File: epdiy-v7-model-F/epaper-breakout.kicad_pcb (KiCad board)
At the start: 4 copper layers, 100 x 55 mm, 111 parts, among them J2 EXTENSION_HEADER, J3 SM04B-SRSS-TB_LF__SN_, J4 XF2M-3315-1A, J5 CONN_BAT, J6 8BIT_HEADER, J7 ESP_HDR, J8 ED133UT2, J9 USB_C_Receptacle_USB2.0, Q1 AO3401A, U1 MCP1700-3302E_SOT23, U10 RT9080-33GJ5, U11 TP4056, U2 PCA9535PW, U3 TPS651851RSLR, U6 ED078KH6, U8 ESP32-S3-WROOM-1, Y1 RV-3032-C7

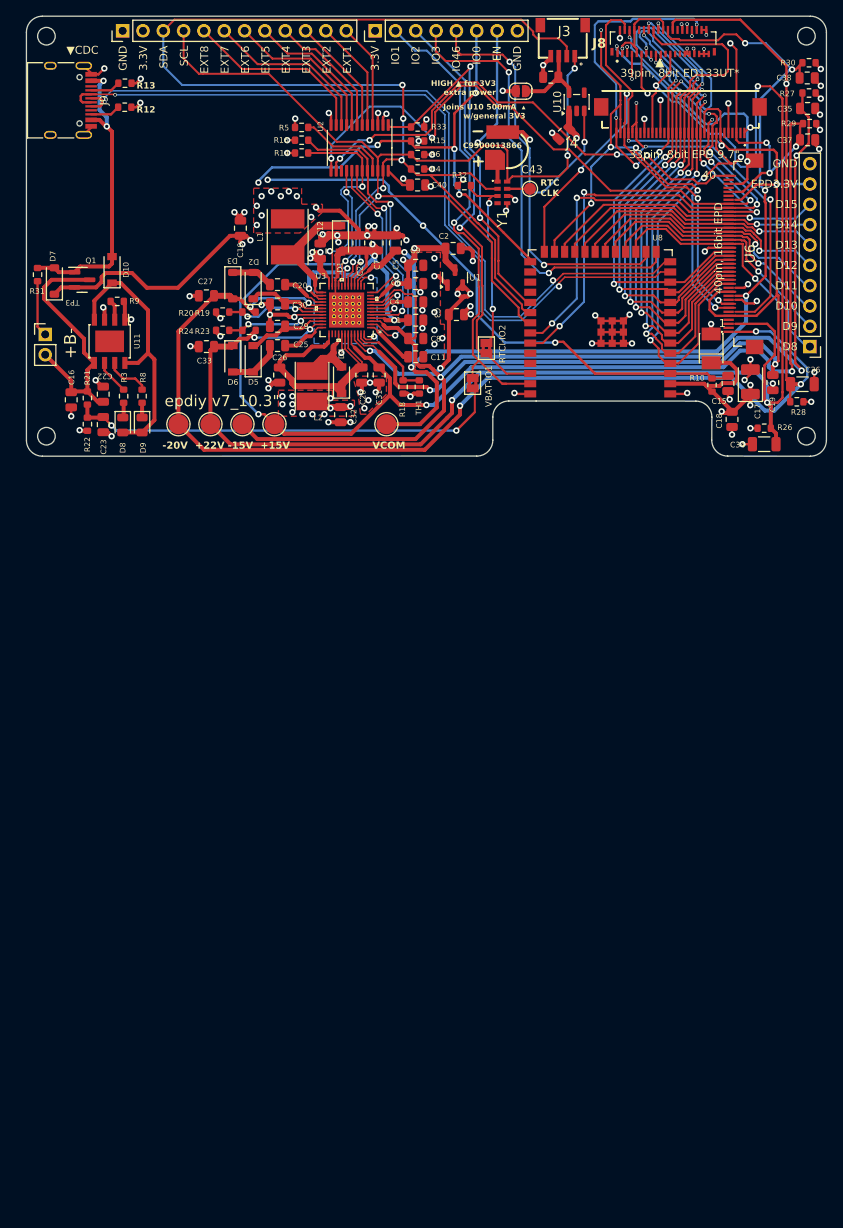
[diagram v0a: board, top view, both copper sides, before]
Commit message: Starting to accomodate stuff over the board
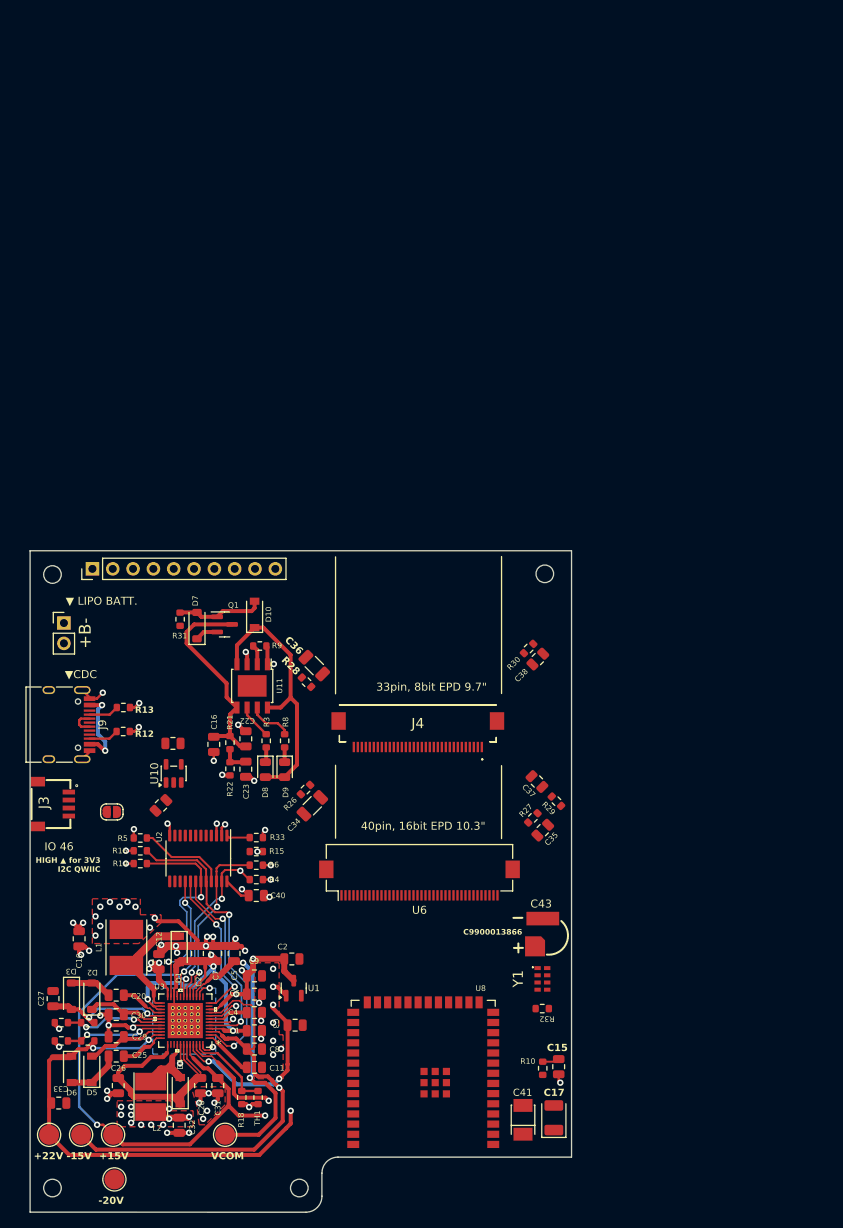
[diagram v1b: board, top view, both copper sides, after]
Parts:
- removed C18: 1uF, Capacitor_SMD:C_0805_2012Metric
- removed C19: 10uF, Capacitor_SMD:C_0805_2012Metric
- removed J2: EXTENSION_HEADER, Connector_PinHeader_2.54mm:PinHeader_1x12_P2.54mm_Vertical
- removed J7: ESP_HDR, Connector_PinHeader_2.54mm:PinHeader_1x08_P2.54mm_Vertical
- removed J8: ED133UT2, epaper-breakout:HRS_FH26W-39S-0.3SHW(60)
- removed JP1: VBAT_GPIO2, Jumper:SolderJumper-2_P1.3mm_Bridged2Bar_Pad1.0x1.5mm
- removed JP2: RTCINT_GPIO2, Jumper:SolderJumper-2_P1.3mm_Bridged2Bar_Pad1.0x1.5mm
- removed TP6: RTC_CLK, TestPoint:TestPoint_Pad_D1.5mm
- U6: footprint footprints:FH1240S05SH55 -> epaper-breakout:Hirose_FH12-40S-0.5SH_mirrored
- moved J3 117.8 mm to (22.5, 115.4), turned to -90 degrees
- moved H3 113.4 mm to (56.0, 166.4)
- moved JP3 103.6 mm to (32.5, 119.4)
- moved R32 103.3 mm to (86.3, 144.0), turned to 0 degrees
- moved C41 99.3 mm to (83.9, 157.9)
- moved Y1 98.4 mm to (86.4, 140.3)
- moved C43 98.4 mm to (85.9, 134.7)
- moved C21 97.9 mm to (38.7, 118.6)
- moved U10 97.9 mm to (40.3, 114.6)
- moved R27 97.0 mm to (85.2, 120.1), turned to 45 degrees
- moved U8 96.4 mm to (71.5, 152.7)
- moved C33 96.3 mm to (25.9, 155.8), turned to 0 degrees
- moved C35 96.1 mm to (86.4, 121.7), turned to 45 degrees
- moved C39 95.7 mm to (40.2, 110.8), turned to 180 degrees
- moved C17 95.2 mm to (87.8, 157.6)
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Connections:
- U2 pad 10: /EXT7 -> unconnected-(U2-IO0_6-Pad10)
- U2 pad 11: /EXT8 -> unconnected-(U2-IO0_7-Pad11)
- U2 pad 4: /EXT1 -> unconnected-(U2-IO0_0-Pad4)
- U2 pad 5: /EXT2 -> unconnected-(U2-IO0_1-Pad5)
- U2 pad 6: /EXT3 -> unconnected-(U2-IO0_2-Pad6)
- U2 pad 7: /EXT4 -> unconnected-(U2-IO0_3-Pad7)
- U2 pad 8: /EXT5 -> unconnected-(U2-IO0_4-Pad8)
- U2 pad 9: /EXT6 -> unconnected-(U2-IO0_5-Pad9)
- U8 pad 10: /D5 -> /D10
- U8 pad 11: /D6 -> /D9
- U8 pad 12: /D7 -> /D8
- U8 pad 17: /D8 -> /D7
- U8 pad 18: /D9 -> /D6
- U8 pad 19: /D10 -> /D5
- U8 pad 20: /D11 -> /D4
- U8 pad 21: /D12 -> /D3
- U8 pad 22: /D13 -> /D2
- U8 pad 23: /D14 -> /D1
- U8 pad 24: /D15 -> /D0
- U8 pad 25: /CKV -> /LEH
- U8 pad 26: /EP_STV -> /XSTL
- U8 pad 31: /~{GPIO_INTR} -> /GPIO_38
- U8 pad 34: /XSTL -> /EP_STV
- U8 pad 35: /LEH -> /CKV
- U8 pad 38: /GPIO_2 -> /~{GPIO_INTR}
- U8 pad 5: /D0 -> /D15
- U8 pad 6: /D1 -> /D14
- U8 pad 7: /D2 -> /D13
- U8 pad 8: /D3 -> /D12
- U8 pad 9: /D4 -> /D11
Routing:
- net /-20V: track 216.9 -> 16.2 mm, vias 7 -> 2
- net EPD_VDD: track 161.4 -> 13.5 mm, vias 5 -> 1
- net /+22V: track 206.1 -> 60.3 mm, vias 6 -> 3
- net /SDA: track 155.1 -> 22.1 mm, vias 5 -> 3
- net /15V: track 200.4 -> 69.3 mm, vias 9 -> 3
- net /EP_VCOM: track 165.1 -> 38.3 mm, vias 7 -> 2
- net /-15V: track 181.8 -> 57.3 mm, vias 6 -> 1
- net /EP_MODE: track 109.2 -> 0.00 mm, vias 7 -> 0
- net /ESP_USB+: track 101.9 -> 0.00 mm, vias 2 -> 0
- net /SCL: track 123.6 -> 21.9 mm, vias 4 -> 2
- net /EP_OE: track 99.8 -> 0.00 mm, vias 6 -> 0
- net /ESP_USB-: track 101.9 -> 3.33 mm, vias 2 -> 0
- net /EN: track 99.2 -> 2.13 mm, vias 4 -> 0
- net GND: track 189.1 -> 94.0 mm, vias 104 -> 64
- net /CKV: track 81.8 -> 0.00 mm, vias 7 -> 0
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- removed copper zone on In2.Cu, net 3.3V
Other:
- board size 100 x 55 mm -> 67.7 x 82.7 mm
- board text added: "40pin, 16bit EPD 10.3{dblquote}"
- board text added: "HIGH ▲ for 3V3 I2C QWIIC"
- board text added: "IO 46"
- board text added: "▼ LIPO BATT."
- board text removed: "1"
- board text removed: "3.3V"
- board text removed: "39pin, 8bit ED133UT*"
- board text removed: "40"
- board text removed: "40pin, 16bit EPD"
- board text removed: "D10"
- board text removed: "D11"
- board text removed: "D12"
- board text removed: "D13"
- board text removed: "D14"
- board text removed: "D15"
- board text removed: "D8"
- board text removed: "D9"
- board text removed: "EN"
- board text removed: "EPD3.3V"
- board text removed: "EXT1"
- board text removed: "EXT2"
- board text removed: "EXT3"
- board text removed: "EXT4"
- board text removed: "EXT5"
- board text removed: "EXT6"
- board text removed: "EXT7"
- board text removed: "EXT8"
- board text removed: "GND"
- board text removed: "HIGH ▲ for 3V3 extra power"
- board text removed: "IO0"
- board text removed: "IO1"
- board text removed: "IO2"
- board text removed: "IO3"
- board text removed: "IO46"
- board text removed: "Joins U10 500mA ▴ w/general 3V3"
- board text removed: "RTC CLK"
- board text removed: "RTCI-IO2"
- board text removed: "Rel 1.1.1 PCB custom modified for 9.7, 13.3 inch displays (8 bit)"
- board text removed: "SCL"
- board text removed: "SDA"
- board text removed: "VBAT-IO1"
- board text removed: "epdiy v7 by Valentin Roland 2023 Thanks to the epdiy contributors! For sources and documentation visit https://github.com/vroland/epdiy"
- board text removed: "epdiy v7_10.3{dblquote}"
- board text removed: "▲"
